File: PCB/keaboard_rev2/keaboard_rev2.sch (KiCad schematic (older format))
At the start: 88 parts, among them J1 AudioJack4, P1 OLED, P2 LED, SW1 SW_Push, SW10 SW_Push, SW11 SW_Push, SW12 SW_Push, SW13 SW_Push, SW14 SW_Push, SW15 SW_Push, SW16 SW_Push, SW17 SW_Push, SW18 SW_Push, SW19 SW_Push, SW2 SW_Push, SW20 SW_Push, SW21 SW_Push, SW22 SW_Push, SW23 SW_Push, SW24 SW_Push, SW25 SW_Push, SW3 SW_Push, SW4 SW_Push, SW5 SW_Push, SW6 SW_Push, SW7 SW_Push, SW8 SW_Push, SW9 SW_Push, U1 ProMicro

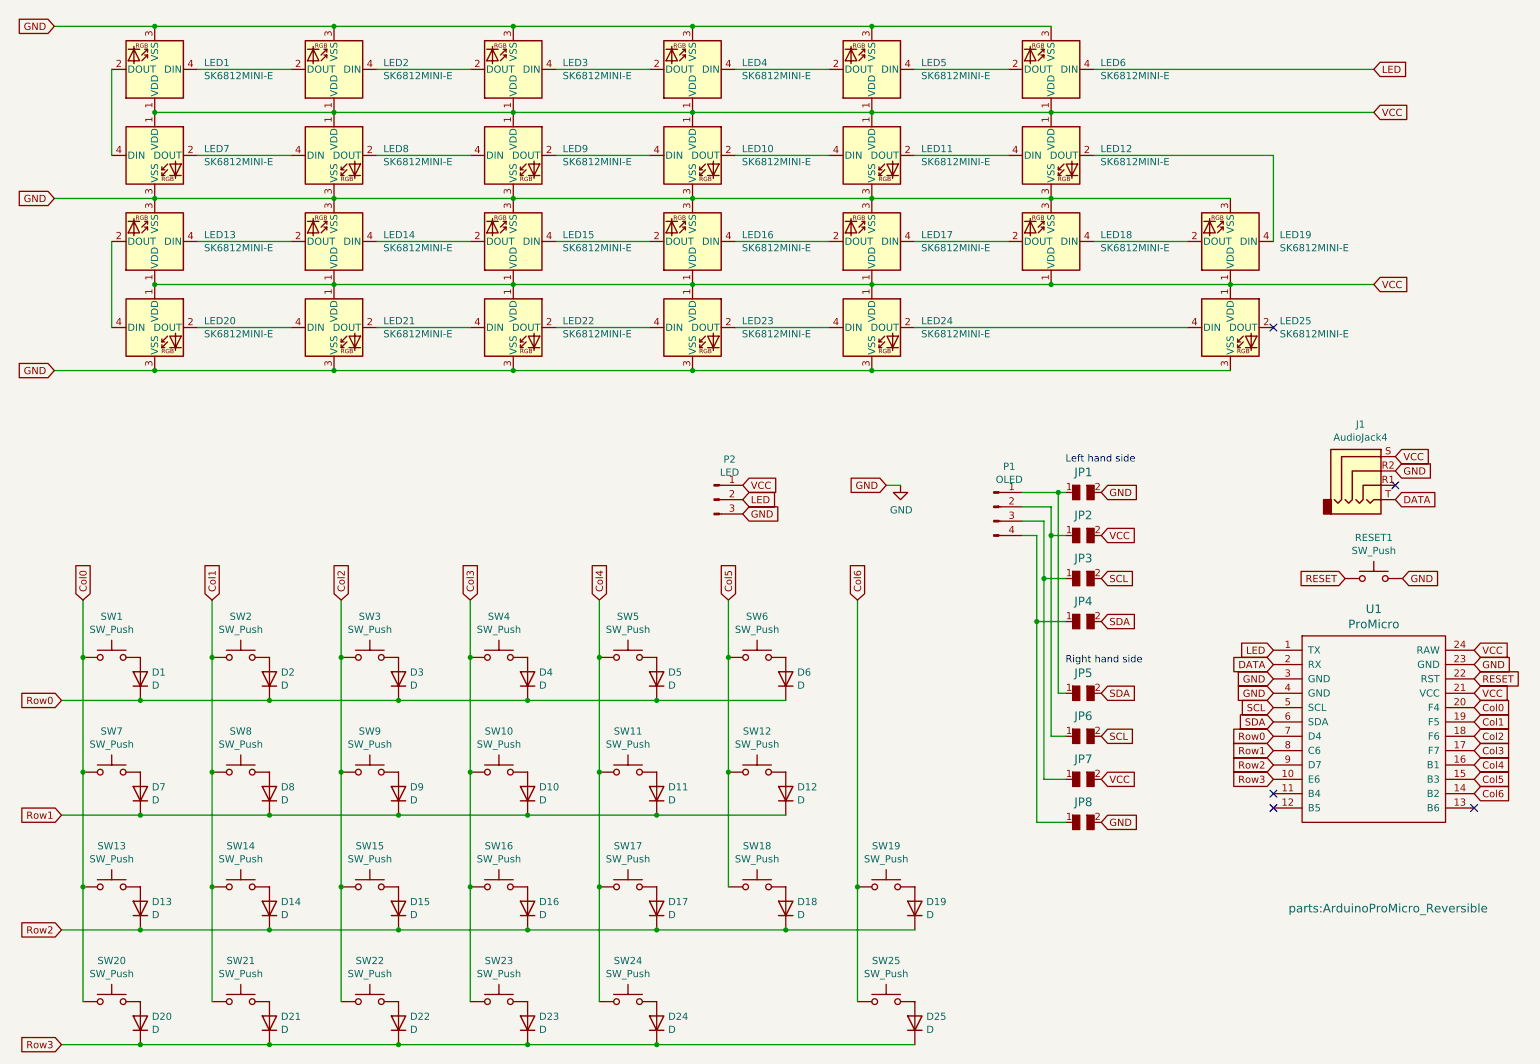
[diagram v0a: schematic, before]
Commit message: WIP
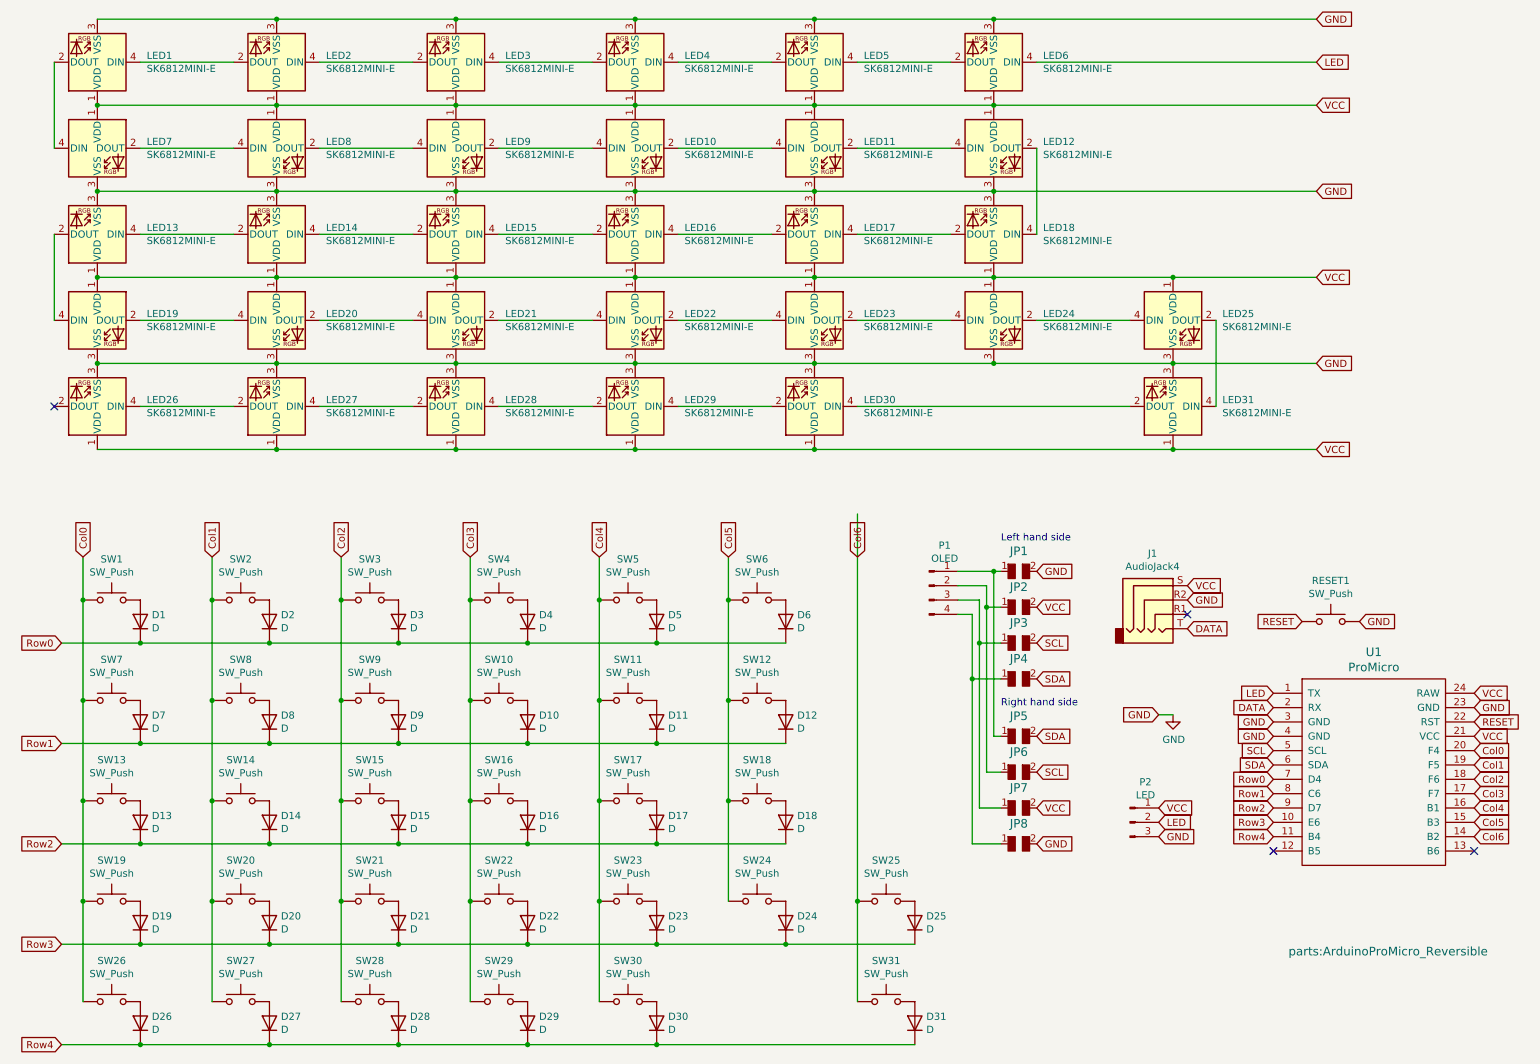
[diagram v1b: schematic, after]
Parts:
- removed LED19: SK6812MINI-E, parts:SK6812MINI-E_reversible, symbol kicad-keyboard-parts:SK6812MINI-E
- added D13, D14, D15, D16, D17, D18: D, Keebio-Parts:Diode-dual, symbol Diode:1N4148W
- added LED25, LED26, LED27, LED28, LED29, LED30, LED31: SK6812MINI-E, parts:SK6812MINI-E_reversible, symbol kicad-keyboard-parts:SK6812MINI-E
- added SW13, SW14, SW15, SW16, SW17, SW18: SW_Push, keyswitches:Kailh_socket_PG1350_reversible, symbol Switch:SW_Push
- renumbered D13 to D19, D14 to D20, D15 to D21, D16 to D22, D17 to D23, D18 to D24, D19 to D25, D20 to D26, D21 to D27, D22 to D28, D23 to D29, D24 to D30, D25 to D31, LED20 to LED19, LED21 to LED20, LED22 to LED21, LED23 to LED22, LED24 to LED23, LED25 to LED24, SW13 to SW19, SW14 to SW20, SW15 to SW21, SW16 to SW22, SW17 to SW23, SW18 to SW24, SW19 to SW25, SW20 to SW26, SW21 to SW27, SW22 to SW28, SW23 to SW29, SW24 to SW30, SW25 to SW31
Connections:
- net Col0: now also SW13.1
- net Col1: now also SW14.1
- net Col2: now also SW15.1
- net Col3: now also SW16.1
- net Col4: now also SW17.1
- net Col5: now also SW18.1
- net GND: now also LED25.3 (VSS), LED26.3 (VSS), LED27.3 (VSS), LED28.3 (VSS), LED29.3 (VSS), LED30.3 (VSS), LED31.3 (VSS)
- net Row2: now also D13.1 (K), D14.1 (K), D15.1 (K), D16.1 (K), D17.1 (K), D18.1 (K); no longer D19.1 (K), D20.1 (K), D21.1 (K), D22.1 (K), D23.1 (K), D24.1 (K), D25.1 (K)
- net Row3: now also D19.1 (K), D20.1 (K), D21.1 (K), D22.1 (K), D23.1 (K), D24.1 (K), D25.1 (K); no longer D26.1 (K), D27.1 (K), D28.1 (K), D29.1 (K), D30.1 (K), D31.1 (K)
- net VCC: now also LED25.1 (VDD), LED26.1 (VDD), LED27.1 (VDD), LED28.1 (VDD), LED29.1 (VDD), LED30.1 (VDD), LED31.1 (VDD)
- net Row4: now reaches U1.11 (B4)
- net Row4: now also D26.1 (K), D27.1 (K), D28.1 (K), D29.1 (K), D30.1 (K), D31.1 (K)
- net at LED12.2 (DOUT): now also LED18.4 (DIN)
- net at LED24.2 (DOUT): now also LED25.4 (DIN)
- new net: D18.2 (A), SW18.2
- new net: D17.2 (A), SW17.2
- new net: D16.2 (A), SW16.2
- new net: D15.2 (A), SW15.2
- new net: D14.2 (A), SW14.2
- new net: D13.2 (A), SW13.2
- new net: LED25.2 (DOUT), LED31.4 (DIN)
- new net: LED26.4 (DIN), LED27.2 (DOUT)
- new net: LED27.4 (DIN), LED28.2 (DOUT)
- new net: LED28.4 (DIN), LED29.2 (DOUT)
- new net: LED29.4 (DIN), LED30.2 (DOUT)
- new net: LED30.4 (DIN), LED31.2 (DOUT)
- no-connect marks 5 -> 4
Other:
- moved on the sheet: D1, D10, D11, D12, D19, D2, D20, D21, D22, D23, D24, D25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
